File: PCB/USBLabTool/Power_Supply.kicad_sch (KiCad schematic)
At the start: 53 parts, among them J19 T_N5V, U10 Opamp_Quad, U11 DG403, U13 r1283, U14 ST1L05APU33R, U15 ST1L05APU33R, U16 LTC1983ES6-5#TRPBF, U9 Opamp_Quad

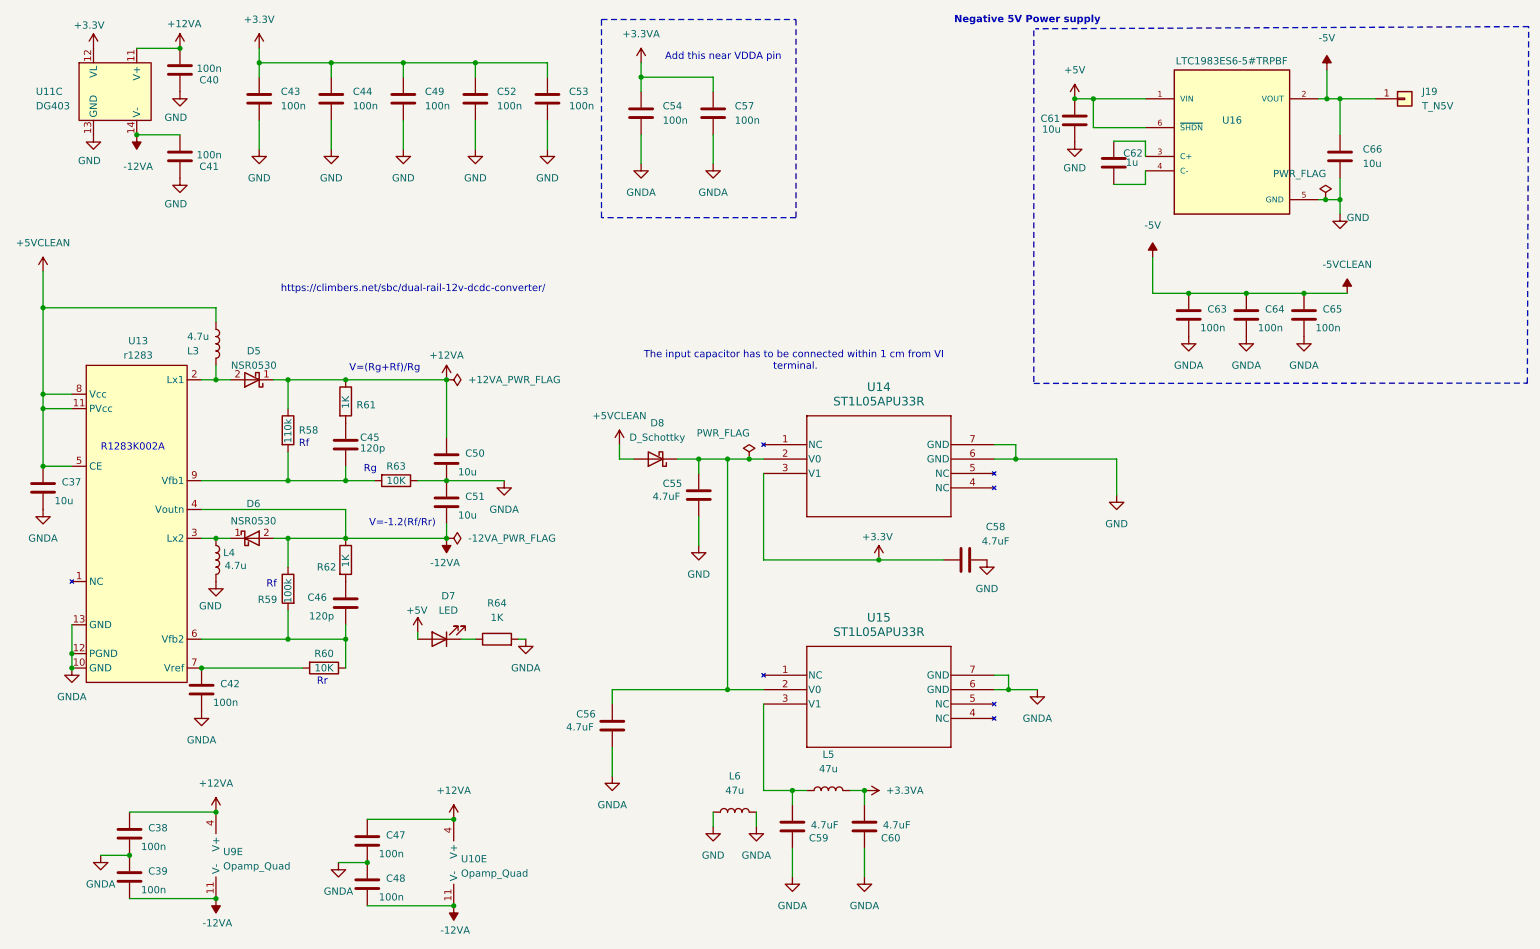
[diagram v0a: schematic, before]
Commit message: Update Power_Supply.kicad_sch
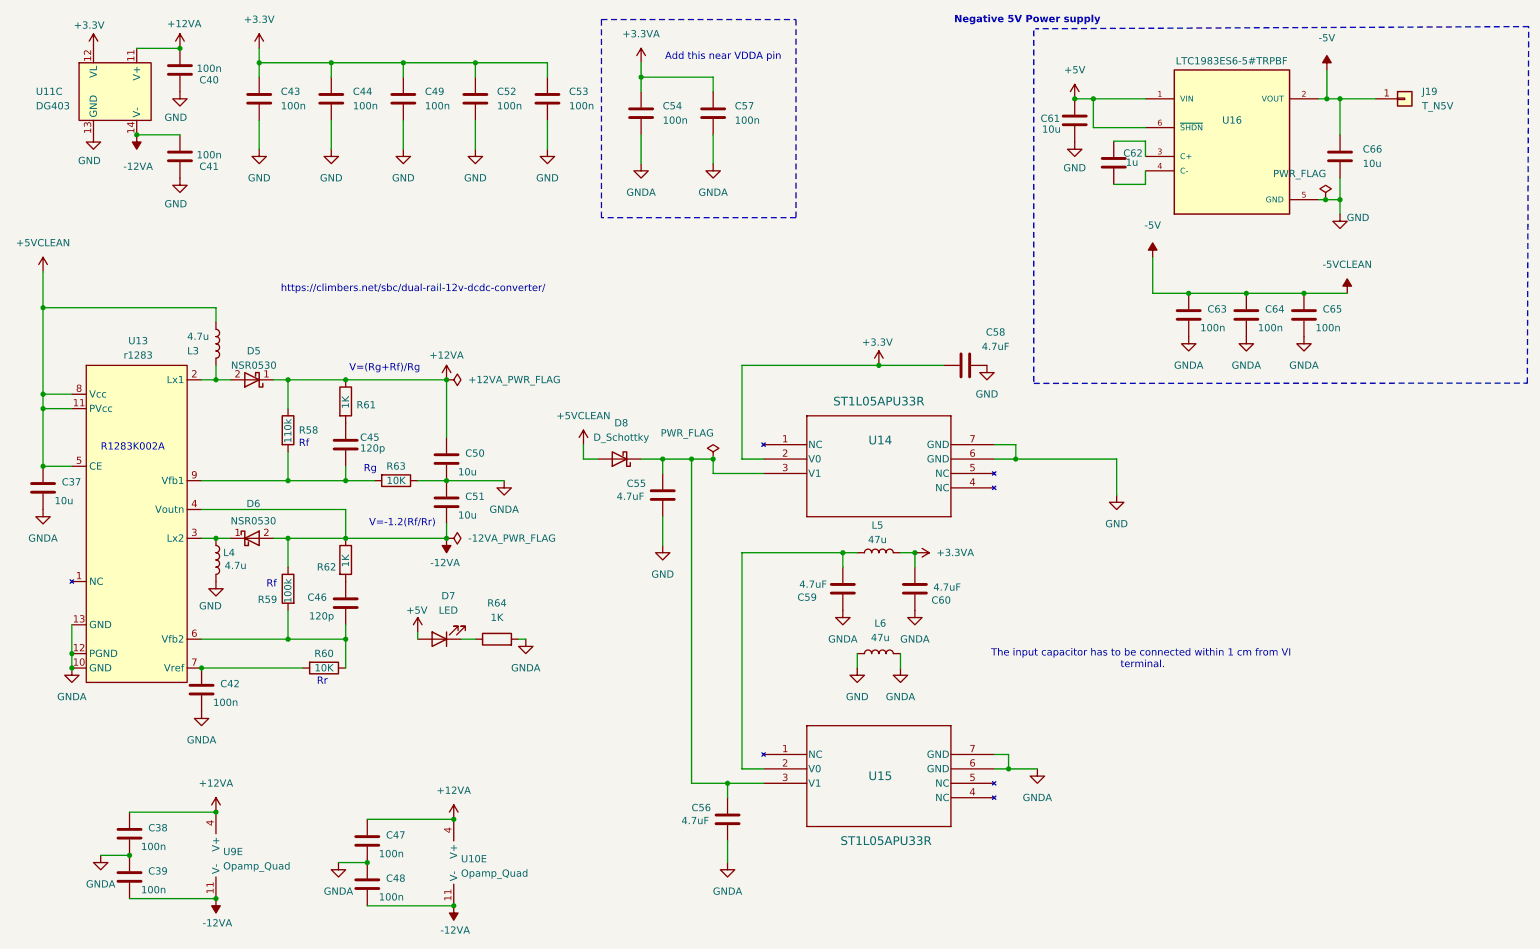
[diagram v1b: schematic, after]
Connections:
- net +3.3V: now also U14.2 (V0); no longer U14.3 (V1)
- net at C59.2, L5.1: now also U15.2 (V0); no longer U15.3 (V1)
- net at C55.1, C56.1, D8.1 (K): now also U14.3 (V1), U15.3 (V1); no longer U14.2 (V0), U15.2 (V0)
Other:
- moved on the sheet: C55, C56, C58, C59, C60, D8, L5, L6, U15
